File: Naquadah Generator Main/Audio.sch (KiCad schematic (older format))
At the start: 48 parts, among them U10 PAM8302AAD, U7 VS1000, U9 MX25L1606EM1I-12G, Y2 12MHz

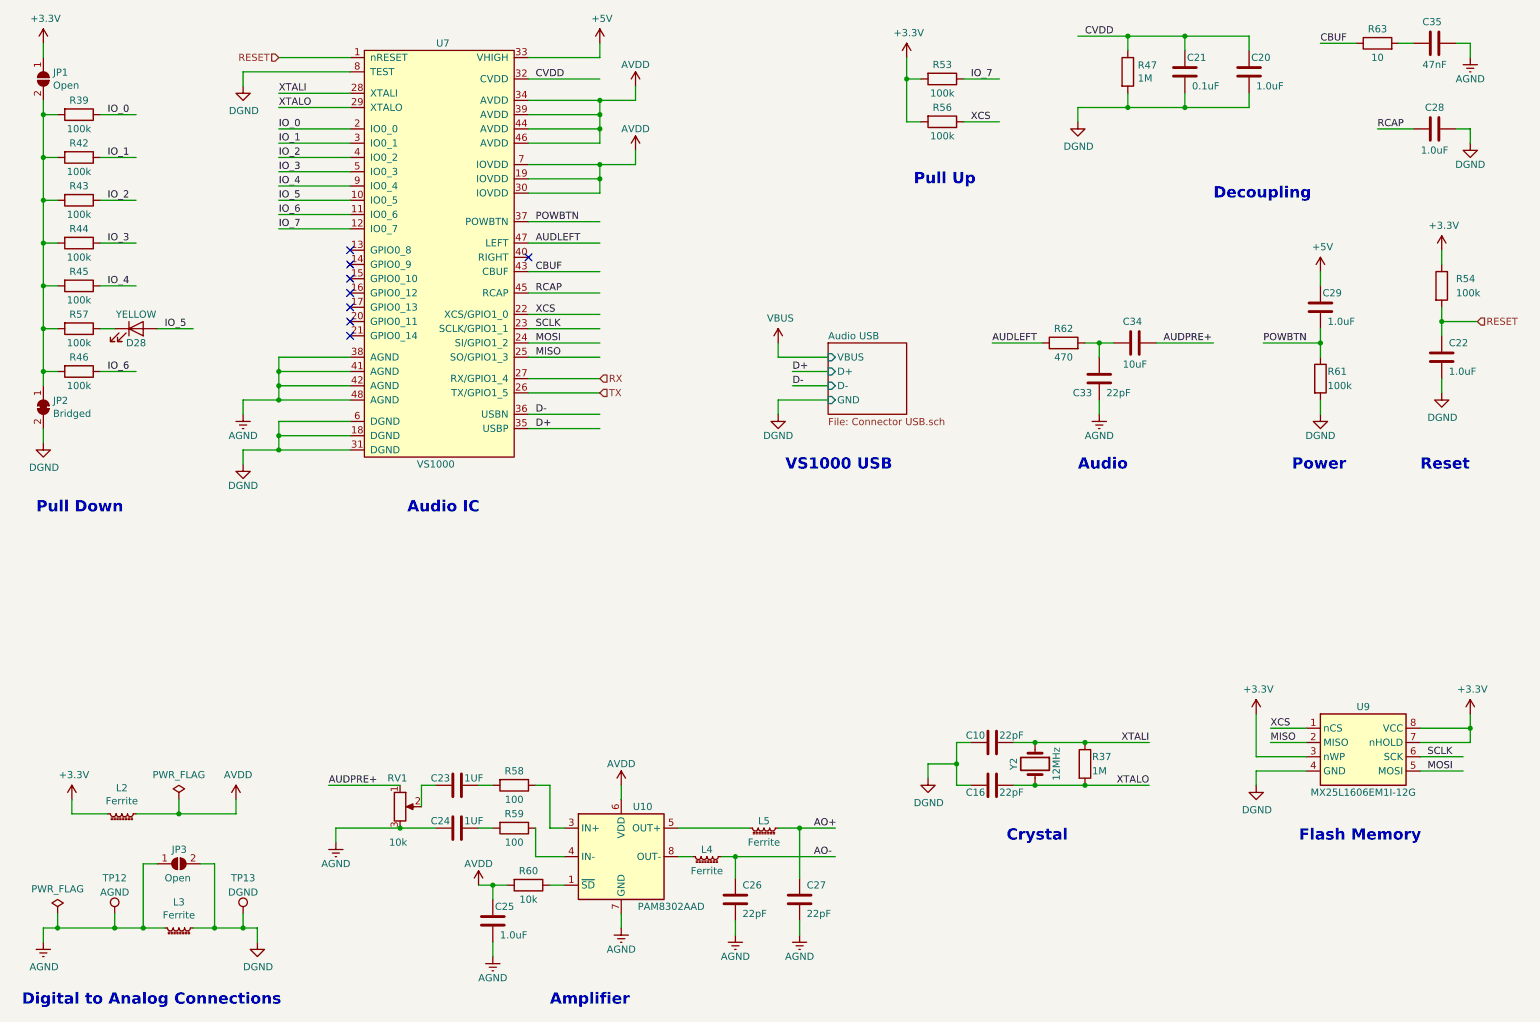
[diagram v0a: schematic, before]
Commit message: Added level shifter, moved user interface connector location
Added level shifter, moved user interface connector location
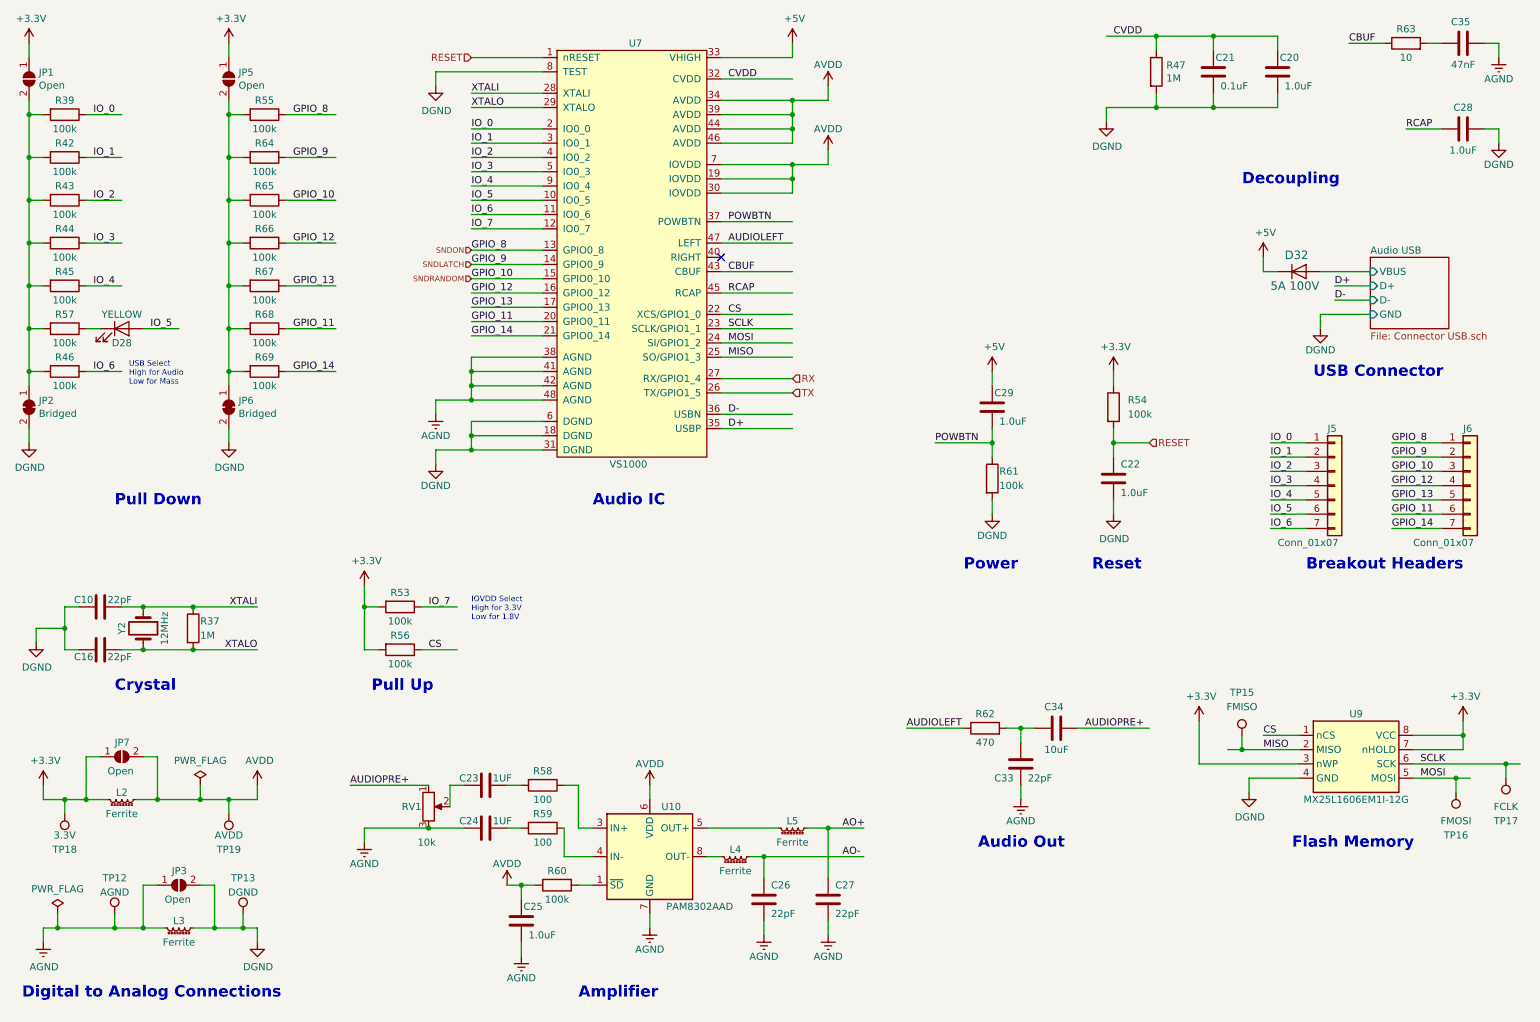
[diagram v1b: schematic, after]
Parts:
- added D32: 5A 100V, Li_Ion_LE:DO-214AC, symbol Frequently_Used_LE:D
- added J5, J6: Conn_01x07, Connectors_LE:Header_1x07_P2.54mm_Surface, symbol Connector_Generic:Conn_01x07
- added JP5, JP7: Open, Jumper_LE:SolderJumper-2_P1.3mm_Open_RoundedPad1.0x1.5mm, symbol Jumper:SolderJumper_2_Open
- added JP6: Bridged, Jumper_LE:SolderJumper-2_P1.3mm_Bridged_RoundedPad1.0x1.5mm, symbol Jumper:SolderJumper_2_Bridged
- added R55, R64, R65, R66, R67, R68, R69: 100k, Frequently_Used_LE:0603_1608Metric, symbol Frequently_Used_LE:R
- added TP15, TP16, TP17, TP18, TP19: TestPoint, Frequently_Used_LE:Pad_2.5-2.5, symbol Frequently_Used_LE:TestPoint_1
- C20, C22, C25, C28, C29: Description (none) -> 1µF ±10% 16V Ceramic Capacitor X7R 0805 (2012 Metric); Manufacturer Name (none) -> Samsung Electro-Mechanics; Manufacturer Part No. (none) -> CL21B105KOFNNWE; Source Part No. (none) -> 1276-2931-1-ND
- R37, R47, R62, R63: footprint Frequently_Used_LE:0805_2012Metric_HandSolder -> Frequently_Used_LE:0805_2012Metric
- R39, R42, R43, R44, R45, R46, R53, R54, R56, R57, R61: footprint Frequently_Used_LE:0805_2012Metric_HandSolder -> Frequently_Used_LE:0603_1608Metric; Description 100 kOhms ±1% 0.25W, 1/4W Chip Resistor 0805 (2012 Metric) -> 1 kOhms ±1% 0.125W, 1/8W Chip Resistor 0603 (1608 Metric) A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; Manufacturer Part No. RK73H2ATTD1003F -> RK73H1JTTD1001F; Source Part No. 2019-RK73H2ATTD1003FCT-ND -> 2019-RK73H1JTTD1001FCT-ND
- R58, R59: footprint Frequently_Used_LE:0805_2012Metric_HandSolder -> Frequently_Used_LE:0805_2012Metric; Description 100 kOhms ±1% 0.25W, 1/4W Chip Resistor 0805 (2012 Metric) -> 100 Ohms ±1% 0.25W, 1/4W Chip Resistor 0805 (2012 Metric) A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; Manufacturer Part No. RK73H2ATTD1003F -> RK73H2ATTD1000F; Source Part No. 2019-RK73H2ATTD1003FCT-ND -> 2019-RK73H2ATTD1000FCT-ND
- R60: value 10k -> 100k; footprint Frequently_Used_LE:0805_2012Metric_HandSolder -> Frequently_Used_LE:0603_1608Metric; Description 100 kOhms ±1% 0.25W, 1/4W Chip Resistor 0805 (2012 Metric) -> 1 kOhms ±1% 0.125W, 1/8W Chip Resistor 0603 (1608 Metric) A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; Manufacturer Part No. RK73H2ATTD1003F -> RK73H1JTTD1001F; Source Part No. 2019-RK73H2ATTD1003FCT-ND -> 2019-RK73H1JTTD1001FCT-ND
- U9: Description (none) -> FLASH - NOR Memory IC 16Mb (2M x 8) SPI 86MHz 8-SOP; Manufacturer Name (none) -> Macronix; Manufacturer Part No. (none) -> MX25L1606EM1I-12G; Source (none) -> Digikey; Source Part No. (none) -> 1092-1122-ND
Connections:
- net labels added: AUDIOLEFT, AUDIOPRE+, CS, GPIO_10, GPIO_11, GPIO_12, GPIO_13, GPIO_14, GPIO_8, GPIO_9, SNDLATCH, SNDON, SNDRANDOM
- net labels removed: AUDLEFT, AUDPRE+, VBUS, XCS
- wire segments 209 -> 271
- no-connect marks 8 -> 1
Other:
- note added: "Audio Out"
- note added: "Breakout Headers"
- note added: "IOVDD Select\nHigh for 3.3V\nLow for 1.8V"
- note added: "USB Connector"
- note added: "USB Select\nHigh for Audio\nLow for Mass"
- note removed: "Audio"
- note removed: "VS1000 USB"
- moved on the sheet: C10, C16, C20, C21, C22, C23, C24, C25, C26, C27, C28, C29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

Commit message: Switched to 0603_1608M size for passives
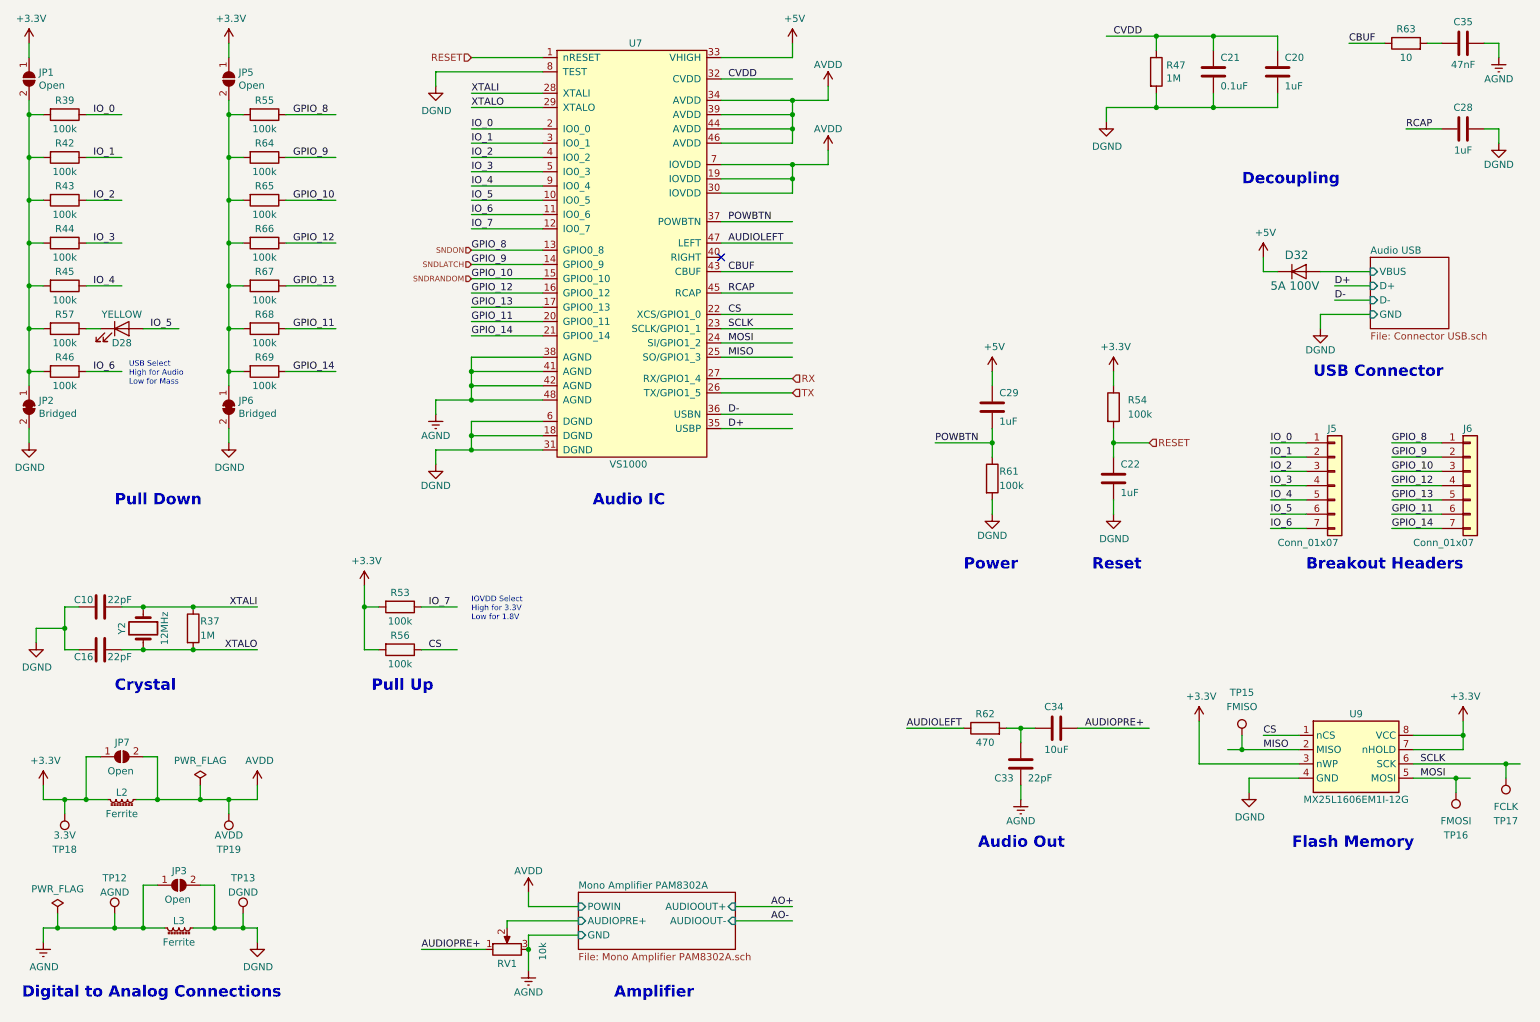
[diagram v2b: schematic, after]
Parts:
- removed C23, C24: 1UF, Frequently_Used_LE:0805_2012Metric_HandSolder, symbol Frequently_Used_LE:C
- removed C25: 1.0uF, Frequently_Used_LE:0805_2012Metric_HandSolder, symbol Frequently_Used_LE:C
- removed C26, C27: 22pF, Frequently_Used_LE:0805_2012Metric_HandSolder, symbol Frequently_Used_LE:C
- removed L4, L5: Ferrite, Frequently_Used_LE:0603_1608Metric, symbol Device:L_Core_Ferrite_Small
- removed R58, R59: 100, Frequently_Used_LE:0805_2012Metric, symbol Frequently_Used_LE:R
- removed R60: 100k, Frequently_Used_LE:0603_1608Metric, symbol Frequently_Used_LE:R
- removed U10: PAM8302AAD, Package_SO:SOP-8_3.9x4.9mm_P1.27mm, symbol Amplifier_Audio_LE:PAM8302AAD
- C10, C16, C33: footprint Frequently_Used_LE:0805_2012Metric_HandSolder -> Frequently_Used_LE:0603_1608Metric; Description (none) -> 22pF ±5% 50V Ceramic Capacitor C0G, NP0 0603 (1608 Metric); Manufacturer Name (none) -> Samsung Electro-Mechanics; Manufacturer Part No. (none) -> CL10C220JB8NNNC; Source Part No. (none) -> 1276-1023-1-ND
- C20, C22, C28, C29: value 1.0uF -> 1uF; footprint Frequently_Used_LE:0805_2012Metric_HandSolder -> Frequently_Used_LE:0603_1608Metric; Description 1µF ±10% 16V Ceramic Capacitor X7R 0805 (2012 Metric) -> 1µF ±10% 10V Ceramic Capacitor X5R 0603 (1608 Metric); Manufacturer Part No. CL21B105KOFNNWE -> CL10A105KP8NNNC; Source Part No. 1276-2931-1-ND -> 1276-1182-1-ND
- C21: footprint Frequently_Used_LE:0805_2012Metric_HandSolder -> Frequently_Used_LE:0603_1608Metric; Description (none) -> 0.1µF -20%, +80% 16V Ceramic Capacitor Y5V (F) 0603 (1608 M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; Manufacturer Name (none) -> Samsung Electro-Mechanics; Manufacturer Part No. (none) -> CL10F104ZO8NNNC; Source Part No. (none) -> 1276-1258-1-ND
- C34: footprint Frequently_Used_LE:0805_2012Metric_HandSolder -> Frequently_Used_LE:0603_1608Metric; Description (none) -> 10µF ±20% 6.3V Ceramic Capacitor X5R 0603 (1608 Metric); Manufacturer Name (none) -> Samsung Electro-Mechanics; Manufacturer Part No. (none) -> CL10A106MQ8NNNC; Source Part No. (none) -> 1276-1119-1-ND
- C35: footprint Frequently_Used_LE:0805_2012Metric_HandSolder -> Frequently_Used_LE:0603_1608Metric; Description (none) -> 0.047µF ±10% 50V Ceramic Capacitor X7R 0603 (1608 Metric); Manufacturer Name (none) -> Samsung Electro-Mechanics; Manufacturer Part No. (none) -> CL10B473KB8NNNC; Source Part No. (none) -> 1276-1063-1-ND
- D28: footprint Frequently_Used_LE:LED_0805_2012Metric_HandSolder -> Frequently_Used_LE:LED_0805_2012Metric
- R37, R47: footprint Frequently_Used_LE:0805_2012Metric -> Frequently_Used_LE:0603_1608Metric; Description 1 MOhms ±1% 0.25W, 1/4W Chip Resistor 0805 (2012 Metric) -> 1 MOhms ±1% 0.1W, 1/10W Chip Resistor 0603 (1608 Metric) Au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; Manufacturer Name KOA Speer Electronics, Inc. -> Stackpole Electronics Inc; Manufacturer Part No. RK73H2ATTD1004F -> Stackpole Electronics Inc; Source Part No. 2019-RK73H2ATTD1004FCT-ND -> RMCF0603FG1M00CT-ND
- R62: footprint Frequently_Used_LE:0805_2012Metric -> Frequently_Used_LE:0603_1608Metric; Description 100 kOhms ±1% 0.25W, 1/4W Chip Resistor 0805 (2012 Metric) -> 470 Ohms ±1% 0.125W, 1/8W Chip Resistor 0603 (1608 Metric) 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; Manufacturer Part No. RK73H2ATTD1003F -> RK73H1JTTD4700F; Source Part No. 2019-RK73H2ATTD1003FCT-ND -> 2019-RK73H1JTTD4700FCT-ND
- R63: footprint Frequently_Used_LE:0805_2012Metric -> Frequently_Used_LE:0603_1608Metric; Description 100 kOhms ±1% 0.25W, 1/4W Chip Resistor 0805 (2012 Metric) -> 10 Ohms ±1% 0.125W, 1/8W Chip Resistor 0603 (1608 Metric) A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; Manufacturer Part No. RK73H2ATTD1003F -> RK73H1JTTD10R0F; Source Part No. 2019-RK73H2ATTD1003FCT-ND -> 2019-RK73H1JTTD10R0FCT-ND
- TP12, TP13, TP15, TP16, TP17, TP18, TP19: Description None -> Test point
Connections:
- wire segments 271 -> 251
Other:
- moved on the sheet: RV1
